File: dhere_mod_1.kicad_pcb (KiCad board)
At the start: 2 copper layers, 73.7 x 40.6 mm, 36 parts, among them J1 Power conn, J2 Input conn, J3 MOTOR, J4 Input conn, J5 Input conn, Q1 BC547, Q2 BC557, Q3 IRF4905, Q4 IRF3205, Q5 IRF4905, Q6 IRF3205, Q7 BC547, Q8 BC557, U1 LM358, U2 4N35, U3 4N35

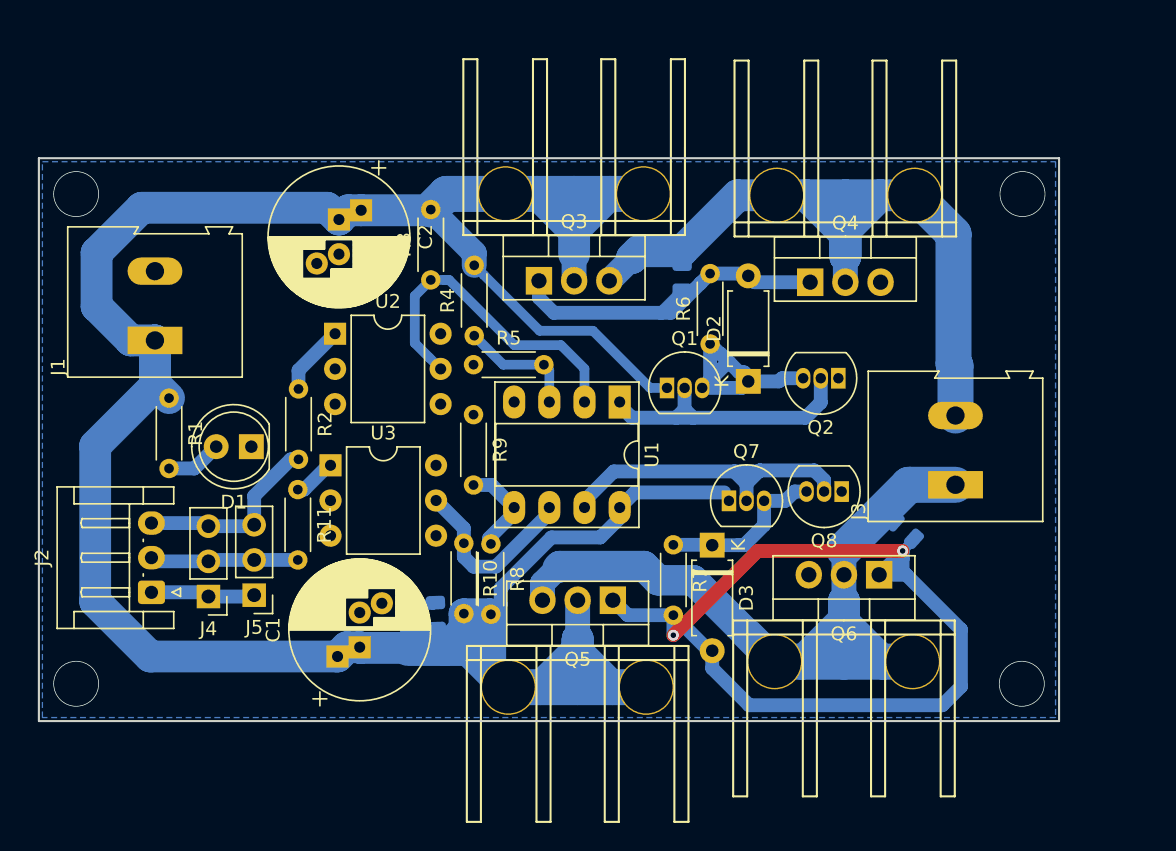
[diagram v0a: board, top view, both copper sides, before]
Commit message: #2 fixed
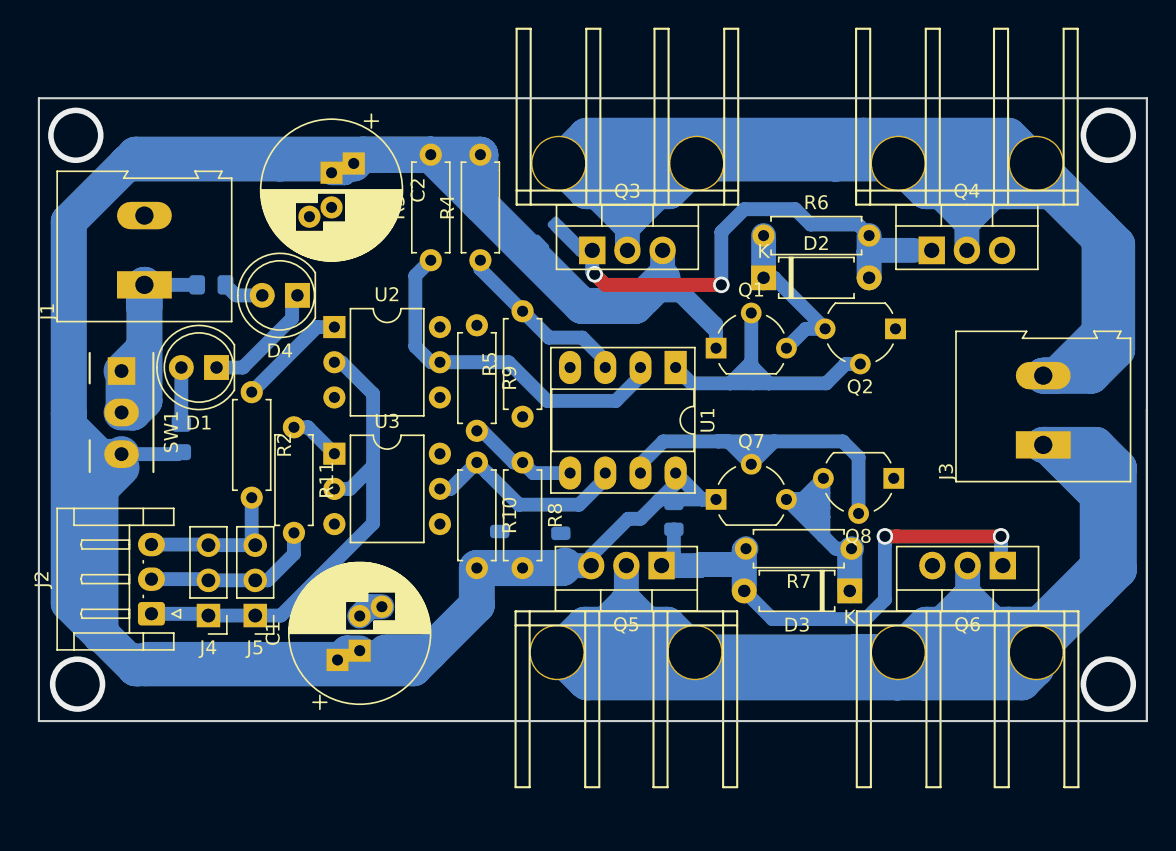
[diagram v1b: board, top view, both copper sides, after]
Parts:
- added D4: LED, LED_THT:LED_D5.0mm_FlatTop, F.Cu at (74.5, 75.9)
- added R12: 5k, Resistor_SMD:R_0805_2012Metric_Pad1.15x1.40mm_HandSolder, B.Cu at (68.3, 75.2)
- added SW1: SW_SPDT, Button_Switch_THT:SW_CuK_OS102011MA1QN1_SPDT_Angled, F.Cu at (61.8, 84.4)
- Q1, Q2, Q7, Q8: footprint Package_TO_SOT_THT:TO-92_Inline -> Package_TO_SOT_THT:TO-92_Wide
- Q5: footprint Package_TO_SOT_THT:TO-220-3_Vertical -> kicad-library:TO-220-3_Vertical
- R1: footprint Resistor_THT:R_Axial_DIN0204_L3.6mm_D1.6mm_P5.08mm_Horizontal -> Resistor_SMD:R_0805_2012Metric_Pad1.15x1.40mm_HandSolder; moved to B.Cu
- R10, R11, R2, R3, R4, R5, R6, R7, R8, R9: footprint Resistor_THT:R_Axial_DIN0204_L3.6mm_D1.6mm_P5.08mm_Horizontal -> Resistor_THT:R_Axial_DIN0207_L6.3mm_D2.5mm_P7.62mm_Horizontal
- moved C5 16.7 mm to (101.7, 91.9), turned to 90 degrees
- moved R7 12.9 mm to (114.6, 94.2), turned to 180 degrees
- moved D3 10.5 mm to (114.4, 97.3), turned to 180 degrees
- moved C4 10.3 mm to (93.6, 94.1), turned to 91 degrees
- moved C6 10.1 mm to (92.7, 71.6), turned to 224 degrees
- moved Q4 9.07 mm to (120.3, 72.7)
- moved Q6 8.95 mm to (125.5, 95.5)
- moved R6 8.72 mm to (108.2, 71.6), turned to 0 degrees
- moved C3 8.42 mm to (89.2, 93.9), turned to 90 degrees
- moved D2 7.56 mm to (108.2, 74.7), turned to 0 degrees
- moved J3 6.96 mm to (128.4, 86.7)
- moved R9 6.46 mm to (87.5, 78.1)
- moved R8 6.31 mm to (90.8, 88.0)
- moved D1 6.24 mm to (68.7, 81.2)
- moved R10 5.90 mm to (87.5, 88.0)
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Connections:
- C5 pad 2: Net-(C5-Pad2) -> VCC
- C6 pad 2: Net-(C6-Pad2) -> VCC
- D2 pad 2: Net-(C6-Pad2) -> Net-(C6-Pad1)
- J1 pad 1: VCC -> Net-(J1-Pad1)
- J2 pad 1: GND -> GNDD
- J3 pad 1: Net-(C5-Pad2) -> Net-(J3-Pad1)
- J3 pad 2: Net-(C6-Pad1) -> Net-(J3-Pad2)
- J4 pad 1: GND -> GNDD
- J5 pad 1: GND -> GNDD
- Q3 pad 1: Net-(C6-Pad2) -> Net-(C6-Pad1)
- Q3 pad 2: VCC -> Net-(J3-Pad2)
- Q3 pad 3: Net-(C6-Pad1) -> VCC
- Q4 pad 1: Net-(C6-Pad2) -> Net-(C6-Pad1)
- Q4 pad 2: Net-(C6-Pad1) -> Net-(J3-Pad2)
- Q5 pad 2: VCC -> Net-(J3-Pad1)
- Q5 pad 3: Net-(C5-Pad2) -> VCC
- Q6 pad 2: Net-(C5-Pad2) -> Net-(J3-Pad1)
- R6 pad 2: Net-(C6-Pad2) -> Net-(C6-Pad1)
- U2 pad 2: GND -> GNDD
- U3 pad 2: GND -> GNDD
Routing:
- net Net-(J3-Pad1): track 0.00 -> 211.4 mm
- net Net-(J3-Pad2): track 0.00 -> 162.8 mm
- net Net-(C5-Pad2): track 60.6 -> 0.00 mm
- net VCC: track 205.5 -> 258.7 mm
- net GNDD: track 0.00 -> 35.4 mm
- net Net-(C5-Pad1): track 67.2 -> 38.8 mm
- net Net-(C6-Pad2): track 27.5 -> 0.00 mm
- net Net-(C6-Pad1): track 60.4 -> 38.0 mm, vias 0 -> 2
- net Net-(J1-Pad1): track 0.00 -> 21.2 mm
- net Net-(D3-Pad1): track 12.3 -> 22.0 mm
- net Net-(Q7-Pad2): track 23.6 -> 28.7 mm
- net Net-(D2-Pad1): track 16.8 -> 12.4 mm
- net Net-(R4-Pad1): track 8.75 -> 12.9 mm
- net Net-(D4-Pad2): track 0.00 -> 2.97 mm
- net /in1: track 13.9 -> 11.0 mm
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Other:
- board size 73.7 x 40.6 mm -> 80 x 45 mm
